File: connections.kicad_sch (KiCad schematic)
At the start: 11 parts, among them J1 Conn_01x03_Socket, J10 Conn_01x06_Socket, J11 Conn_01x06_Socket, J2 Conn_01x02_Socket, J3 Conn_01x03_Socket, J4 Conn_01x03_Socket, J5 Conn_01x03_Socket, J6 Conn_01x23_Socket, J7 Conn_01x03_Socket, J8 Conn_01x03_Socket, J9 Conn_01x03_Socket

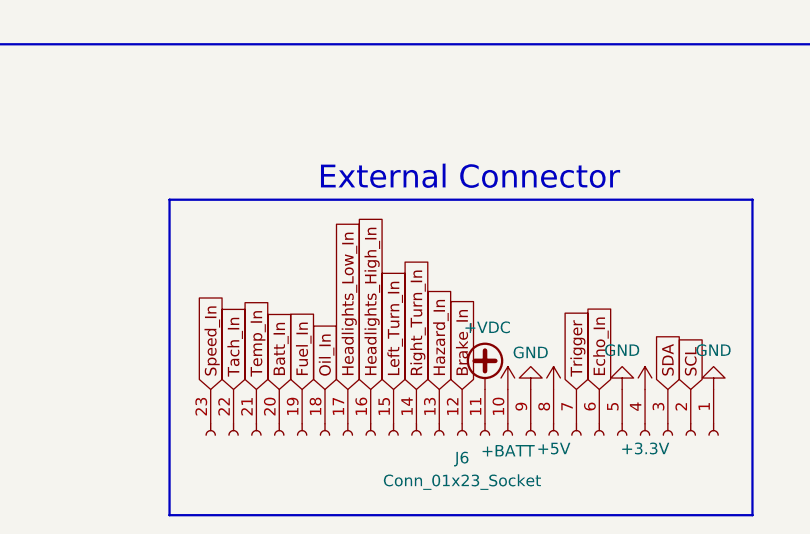
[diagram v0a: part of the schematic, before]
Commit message: Update
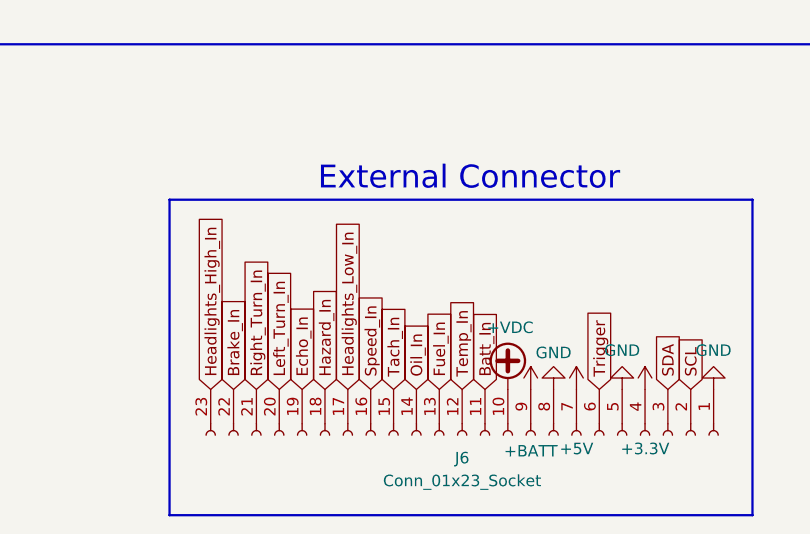
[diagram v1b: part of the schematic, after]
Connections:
- net +5V: now also J6.7 (Pin_7); no longer J6.8 (Pin_8)
- net +BATT: now also J6.9 (Pin_9); no longer J6.10 (Pin_10)
- net +VDC: now also J6.10 (Pin_10); no longer J6.11 (Pin_11)
- net Batt_In: now also J6.11 (Pin_11); no longer J6.20 (Pin_20)
- net Brake_In: now also J6.22 (Pin_22); no longer J6.12 (Pin_12)
- net Echo_In: now also J6.19 (Pin_19); no longer J6.6 (Pin_6)
- net Fuel_In: now also J6.13 (Pin_13); no longer J6.19 (Pin_19)
- net GND: now also J6.8 (Pin_8); no longer J6.9 (Pin_9)
- net Hazard_In: now also J6.18 (Pin_18); no longer J6.13 (Pin_13)
- net Headlights_High_In: now also J6.23 (Pin_23); no longer J6.16 (Pin_16)
- net Left_Turn_In: now also J6.20 (Pin_20); no longer J6.15 (Pin_15)
- net Oil_In: now also J6.14 (Pin_14); no longer J6.18 (Pin_18)
- net Right_Turn_In: now also J6.21 (Pin_21); no longer J6.14 (Pin_14)
- net Speed_In: now also J6.16 (Pin_16); no longer J6.23 (Pin_23)
- net Tach_In: now also J6.15 (Pin_15); no longer J6.22 (Pin_22)
- net Temp_In: now also J6.12 (Pin_12); no longer J6.21 (Pin_21)
- net Trigger: now also J6.6 (Pin_6); no longer J6.7 (Pin_7)
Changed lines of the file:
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@@
 	(global_label "Echo_In"
 		(shape input)
-		(at 158.75 118.11 90)
+		(at 125.73 118.11 90)
 		(fields_autoplaced yes)
 		(effects
@@
 		)
 		(property "Intersheetrefs" "${INTERSHEET_REFS}"
-			(at 158.75 107.8678 90)
+			(at 125.73 107.8678 90)
 			(hide yes)
 			(show_name no)
@@
 	(global_label "Left_Turn_In"
 		(shape input)
-		(at 135.89 118.11 90)
+		(at 123.19 118.11 90)
 		(fields_autoplaced yes)
 		(effects
@@
 		)
 		(property "Intersheetrefs" "${INTERSHEET_REFS}"
-			(at 135.89 103.8159 90)
+			(at 123.19 103.8159 90)
 			(hide yes)
 			(show_name no)
@@
 	(global_label "Right_Turn_In"
 		(shape input)
-		(at 138.43 118.11 90)
+		(at 120.65 118.11 90)
 		(fields_autoplaced yes)
 		(effects
@@
 		)
 		(property "Intersheetrefs" "${INTERSHEET_REFS}"
-			(at 138.43 102.4855 90)
+			(at 120.65 102.4855 90)
 			(hide yes)
 			(show_name no)
@@
 	(global_label "Hazard_In"
 		(shape input)
-		(at 140.97 118.11 90)
+		(at 128.27 118.11 90)
 		(fields_autoplaced yes)
 		(effects
@@
 		)
 		(property "Intersheetrefs" "${INTERSHEET_REFS}"
-			(at 140.97 105.8116 90)
+			(at 128.27 105.8116 90)
 			(hide yes)
 			(show_name no)
@@
 	(global_label "Tach_In"
 		(shape input)
-		(at 118.11 118.11 90)
+		(at 135.89 118.11 90)
 		(fields_autoplaced yes)
 		(effects
@@
 		)
 		(property "Intersheetrefs" "${INTERSHEET_REFS}"
-			(at 118.11 108.0492 90)
+			(at 135.89 108.0492 90)
 			(hide yes)
 			(show_name no)
@@
 	(global_label "Speed_In"
 		(shape input)
-		(at 115.57 118.11 90)
+		(at 133.35 118.11 90)
 		(fields_autoplaced yes)
 		(effects
@@
 		)
 		(property "Intersheetrefs" "${INTERSHEET_REFS}"
-			(at 115.57 106.7187 90)
+			(at 133.35 106.7187 90)
 			(hide yes)
 			(show_name no)
@@
 	(global_label "Fuel_In"
 		(shape input)
-		(at 125.73 118.11 90)
+		(at 140.97 118.11 90)
 		(fields_autoplaced yes)
 		(effects
@@
 		)
 		(property "Intersheetrefs" "${INTERSHEET_REFS}"
-			(at 125.73 108.412 90)
+			(at 140.97 108.412 90)
 			(hide yes)
 			(show_name no)
@@
 	(global_label "Temp_In"
 		(shape input)
-		(at 120.65 118.11 90)
+		(at 143.51 118.11 90)
 		(fields_autoplaced yes)
 		(effects
@@
 		)
 		(property "Intersheetrefs" "${INTERSHEET_REFS}"
-			(at 120.65 107.5049 90)
+			(at 143.51 107.5049 90)
 			(hide yes)
 			(show_name no)
@@
 	(global_label "Brake_In"
 		(shape input)
-		(at 143.51 118.11 90)
+		(at 118.11 118.11 90)
 		(fields_autoplaced yes)
 		(effects
@@
 		)
 		(property "Intersheetrefs" "${INTERSHEET_REFS}"
-			(at 143.51 107.0815 90)
+			(at 118.11 107.0815 90)
 			(hide yes)
 			(show_name no)
@@
 	(global_label "Batt_In"
 		(shape input)
-		(at 123.19 118.11 90)
+		(at 146.05 118.11 90)
 		(fields_autoplaced yes)
 		(effects
@@
 		)
 		(property "Intersheetrefs" "${INTERSHEET_REFS}"
-			(at 123.19 108.533 90)
+			(at 146.05 108.533 90)
 			(hide yes)
 			(show_name no)
@@
 	(global_label "Oil_In"
 		(shape input)
-		(at 128.27 118.11 90)
+		(at 138.43 118.11 90)
 		(fields_autoplaced yes)
 		(effects
@@
 		)
 		(property "Intersheetrefs" "${INTERSHEET_REFS}"
-			(at 128.27 109.8029 90)
+			(at 138.43 109.8029 90)
 			(hide yes)
 			(show_name no)
@@
 	(global_label "Headlights_High_In"
 		(shape input)
-		(at 133.35 118.11 90)
+		(at 115.57 118.11 90)
 		(fields_autoplaced yes)
 		(effects
@@
 		)
 		(property "Intersheetrefs" "${INTERSHEET_REFS}"
-			(at 133.35 97.1636 90)
+			(at 115.57 97.1636 90)
 			(hide yes)
 			(show_name no)
@@
 	(global_label "Trigger"
 		(shape input)
-		(at 156.21 118.11 90)
+		(at 158.75 118.11 90)
 		(fields_autoplaced yes)
 		(effects
@@
 		)
 		(property "Intersheetrefs" "${INTERSHEET_REFS}"
-			(at 156.21 108.5934 90)
+			(at 158.75 108.5934 90)
 			(hide yes)
 			(show_name no)
@@
 	(symbol
 		(lib_id "power:+VDC")
-		(at 146.05 118.11 0)
+		(at 148.59 118.11 0)
 		(unit 1)
 		(body_style 1)
@@
 		(dnp no)
 		(property "Reference" "#PWR031"
-			(at 146.05 120.65 0)
+			(at 148.59 120.65 0)
 			(hide yes)
 			(show_name no)
@@
 		)
 		(property "Value" "+VDC"
-			(at 146.304 111.252 0)
+			(at 148.844 111.252 0)
 			(show_name no)
 			(do_not_autoplace no)
@@
 		)
 		(property "Footprint" ""
-			(at 146.05 118.11 0)
+			(at 148.59 118.11 0)
 			(hide yes)
 			(show_name no)
@@
 		)
 		(property "Datasheet" ""
-			(at 146.05 118.11 0)
+			(at 148.59 118.11 0)
 			(hide yes)
 			(show_name no)
@@
 		)
 		(property "Description" "Power symbol creates a global label with name \"+VDC\""
-			(at 146.05 118.11 0)
+			(at 148.59 118.11 0)
 			(hide yes)
 			(show_name no)
@@
 	(symbol
 		(lib_id "power:+5V")
-		(at 153.67 118.11 0)
+		(at 156.21 118.11 0)
 		(unit 1)
 		(body_style 1)
@@
 		(dnp no)
 		(property "Reference" "#PWR034"
-			(at 153.67 121.92 0)
+			(at 156.21 121.92 0)
 			(hide yes)
 			(show_name no)
@@
 		)
 		(property "Value" "+5V"
-			(at 153.67 124.714 0)
+			(at 156.21 124.714 0)
 			(show_name no)
 			(do_not_autoplace no)
@@
 		)
 		(property "Footprint" ""
-			(at 153.67 118.11 0)
+			(at 156.21 118.11 0)
 			(hide yes)
 			(show_name no)
@@
 		)
 		(property "Datasheet" ""
-			(at 153.67 118.11 0)
+			(at 156.21 118.11 0)
 			(hide yes)
 			(show_name no)
@@
 		)
 		(property "Description" "Power symbol creates a global label with name \"+5V\""
-			(at 153.67 118.11 0)
+			(at 156.21 118.11 0)
 			(hide yes)
 			(show_name no)
@@
 	(symbol
 		(lib_id "power:+BATT")
-		(at 148.59 118.11 0)
+		(at 151.13 118.11 0)
 		(unit 1)
 		(body_style 1)
@@
 		(dnp no)
 		(property "Reference" "#PWR032"
-			(at 148.59 121.92 0)
+			(at 151.13 121.92 0)
 			(hide yes)
 			(show_name no)
@@
 		)
 		(property "Value" "+BATT"
-			(at 148.59 124.968 0)
+			(at 151.13 124.968 0)
 			(show_name no)
 			(do_not_autoplace no)
@@
 		)
 		(property "Footprint" ""
-			(at 148.59 118.11 0)
+			(at 151.13 118.11 0)
 			(hide yes)
 			(show_name no)
@@
 		)
 		(property "Datasheet" ""
-			(at 148.59 118.11 0)
+			(at 151.13 118.11 0)
 			(hide yes)
 			(show_name no)
@@
 		)
 		(property "Description" "Power symbol creates a global label with name \"+BATT\""
-			(at 148.59 118.11 0)
+			(at 151.13 118.11 0)
 			(hide yes)
 			(show_name no)
@@
 	(symbol
 		(lib_id "power:GND")
-		(at 151.13 118.11 180)
+		(at 153.67 118.11 180)
 		(unit 1)
 		(body_style 1)
@@
 		(dnp no)
 		(property "Reference" "#PWR033"
-			(at 151.13 111.76 0)
+			(at 153.67 111.76 0)
 			(hide yes)
 			(show_name no)
@@
 		)
 		(property "Value" "GND"
-			(at 151.13 114.046 0)
+			(at 153.67 114.046 0)
 			(show_name no)
 			(do_not_autoplace no)
@@
 		)
 		(property "Footprint" ""
-			(at 151.13 118.11 0)
+			(at 153.67 118.11 0)
 			(hide yes)
 			(show_name no)
@@
 		)
 		(property "Datasheet" ""
-			(at 151.13 118.11 0)
+			(at 153.67 118.11 0)
 			(hide yes)
 			(show_name no)
@@
 		)
 		(property "Description" "Power symbol creates a global label with name \"GND\" , ground"
-			(at 151.13 118.11 0)
+			(at 153.67 118.11 0)
 			(hide yes)
 			(show_name no)
